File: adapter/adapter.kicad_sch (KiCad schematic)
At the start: 18 parts, among them J1 Conn_01x03_Female, J2 Conn_01x06_Female, SW1 RotaryEncoder_Switch

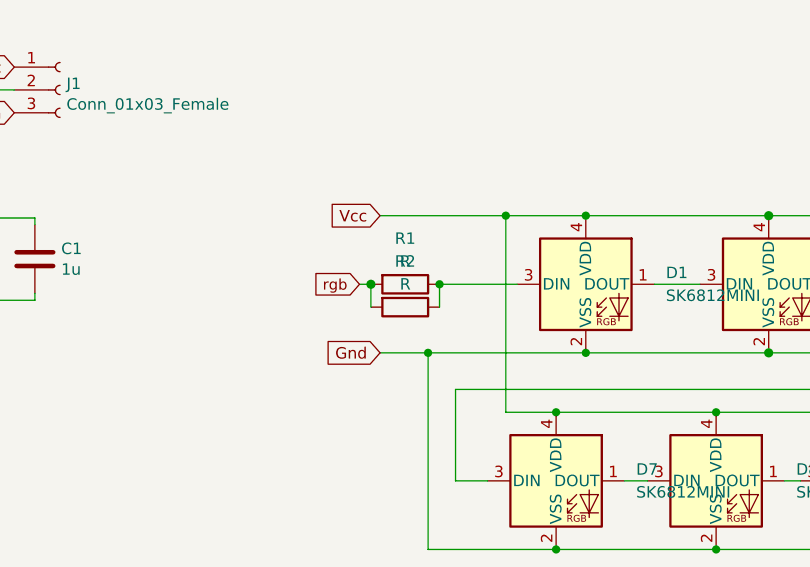
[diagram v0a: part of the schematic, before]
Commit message: routing, add R C
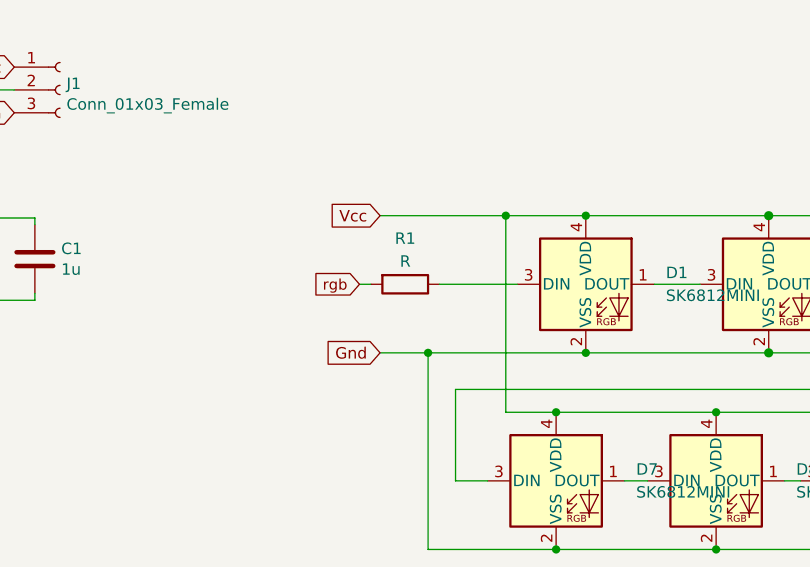
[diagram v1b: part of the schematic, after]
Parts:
- removed R2: R, Resistor_SMD:R_1206_3216Metric_Pad1.42x1.75mm_HandSolder, symbol Device:R
- C1: footprint Capacitor_SMD:C_1206_3216Metric_Pad1.42x1.75mm_HandSolder -> Capacitor_SMD:C_1206_3216Metric_Pad1.33x1.80mm_HandSolder
- R1: footprint Resistor_SMD:R_1206_3216Metric_Pad1.42x1.75mm_HandSolder -> Resistor_SMD:R_1206_3216Metric_Pad1.30x1.75mm_HandSolder
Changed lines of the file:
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@@
   (junction (at 118.11 102.87) (diameter 1.016) (color 0 0 0 0)
   )
-  (junction (at 73.914 95.25) (diameter 1.016) (color 0 0 0 0)
-  )
   (junction (at 30.226 34.29) (diameter 0) (color 0 0 0 0)
   )
@@
   )
   (junction (at 212.09 102.87) (diameter 0) (color 0 0 0 0)
-  )
-  (junction (at 81.534 95.25) (diameter 0) (color 0 0 0 0)
   )
   (junction (at 137.16 87.63) (diameter 0) (color 0 0 0 0)
@@
     (stroke (width 0) (type default) (color 0 0 0 0))
   )
-  (wire (pts (xy 81.534 97.79) (xy 81.534 95.25))
-    (stroke (width 0) (type solid) (color 0 0 0 0))
-  )
   (wire (pts (xy 88.9 87.63) (xy 97.79 87.63))
     (stroke (width 0) (type default) (color 0 0 0 0))
@@
   (wire (pts (xy 112.268 124.714) (xy 129.286 124.714))
     (stroke (width 0) (type default) (color 0 0 0 0))
-  )
-  (wire (pts (xy 73.914 95.25) (xy 73.914 97.79))
-    (stroke (width 0) (type solid) (color 0 0 0 0))
   )
   (wire (pts (xy 112.268 109.474) (xy 129.286 109.474))
@@
     (property "Reference" "R1" (id 0) (at 77.724 90.17 90))
     (property "Value" "R" (id 1) (at 77.724 92.71 90))
-    (property "Footprint" "Resistor_SMD:R_1206_3216Metric_Pad1.42x1.75mm_HandSolder" (id 2) (at 77.724 93.472 90)
+    (property "Footprint" "Resistor_SMD:R_1206_3216Metric_Pad1.30x1.75mm_HandSolder" (id 2) (at 77.724 93.472 90)
       (effects (font (size 1.27 1.27)) hide)
     )
@@
     (pin "1")
   )
-  (symbol (lib_id "Device:R") (at 77.724 97.79 270) (unit 1)
-    (in_bom yes) (on_board yes)
-    (property "Reference" "R2" (id 0) (at 77.724 92.71 90))
-    (property "Value" "R" (id 1) (at 77.724 95.25 90))
-    (property "Footprint" "Resistor_SMD:R_1206_3216Metric_Pad1.42x1.75mm_HandSolder" (id 2) (at 77.724 96.012 90)
-      (effects (font (size 1.27 1.27)) hide)
-    )
-    (property "Datasheet" "~" (id 3) (at 77.724 97.79 0)
-      (effects (font (size 1.27 1.27)) hide)
-    )
-    (pin "1")
-    (pin "2")
-  )
   (symbol (lib_id "power:+5V") (at 30.226 26.67 90) (unit 1)
     (in_bom yes) (on_board yes)
@@
       (effects (font (size 1.27 1.27)) (justify left))
     )
-    (property "Footprint" "Capacitor_SMD:C_1206_3216Metric_Pad1.42x1.75mm_HandSolder" (id 2) (at 37.5412 96.266 0)
+    (property "Footprint" "Capacitor_SMD:C_1206_3216Metric_Pad1.33x1.80mm_HandSolder" (id 2) (at 37.5412 96.266 0)
       (effects (font (size 1.27 1.27)) hide)
     )
@@
     )
     (path "/b720e53b-ae72-4295-b3ff-de5411507232"
-      (reference "C1") (unit 1) (value "1u") (footprint "Capacitor_SMD:C_1206_3216Metric_Pad1.42x1.75mm_HandSolder")
+      (reference "C1") (unit 1) (value "1u") (footprint "Capacitor_SMD:C_1206_3216Metric_Pad1.33x1.80mm_HandSolder")
     )
     (path "/223b04e8-40ea-4e7c-a2bb-67f20935b256"
@@
     )
     (path "/3145c452-dc50-487a-9802-6b13d8b48c50"
-      (reference "R1") (unit 1) (value "R") (footprint "Resistor_SMD:R_1206_3216Metric_Pad1.42x1.75mm_HandSolder")
-    )
-    (path "/890ed13f-42f7-4528-85cf-e8c0911e8d2e"
-      (reference "R2") (unit 1) (value "R") (footprint "Resistor_SMD:R_1206_3216Metric_Pad1.42x1.75mm_HandSolder")
+      (reference "R1") (unit 1) (value "R") (footprint "Resistor_SMD:R_1206_3216Metric_Pad1.30x1.75mm_HandSolder")
     )
     (path "/d31898a0-dde3-4548-9b2f-a263c96d031c"
